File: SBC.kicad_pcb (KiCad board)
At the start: 2 copper layers, 160 x 100.3 mm, 101 parts, among them K1 A17, K10 BNKSEL, K11 16K/32K, K12 INTSEL, K13 RSTSEL, K2 CTS-DSR, K3 RTS-DTR, K4 CTS-DSR, K5 RTS-DTR, K6 A18, K7 128/512, K8 A19, K9 PWR, P1 PARALLEL, P2 POWER, P3 SERIAL, P4 CLK_CPU, P5 CLK_UART, P6 RESET, Q1 2N3906, SW1 RESETSW, U1 16550, U10 74LS243, U11 74LS245, U12 74LS174, U13 74LS174, U14 74LS32, U15 74LS32, U16 74LS32, U17 74LS244, U18 74LS174, U19 8255, U2 27C080, U20 C96ABC, U21 DS1302, U22 MAX232, U23 SRAM_512KO, U24 Z80-CPU, U25 DS1210, U26 74LS06N, U3 74LS08, U4 74LS10, U5 74LS125, U6 74LS139, U7 74LS14, U8 74LS245, U9 74LS245, X1 CRYSTAL

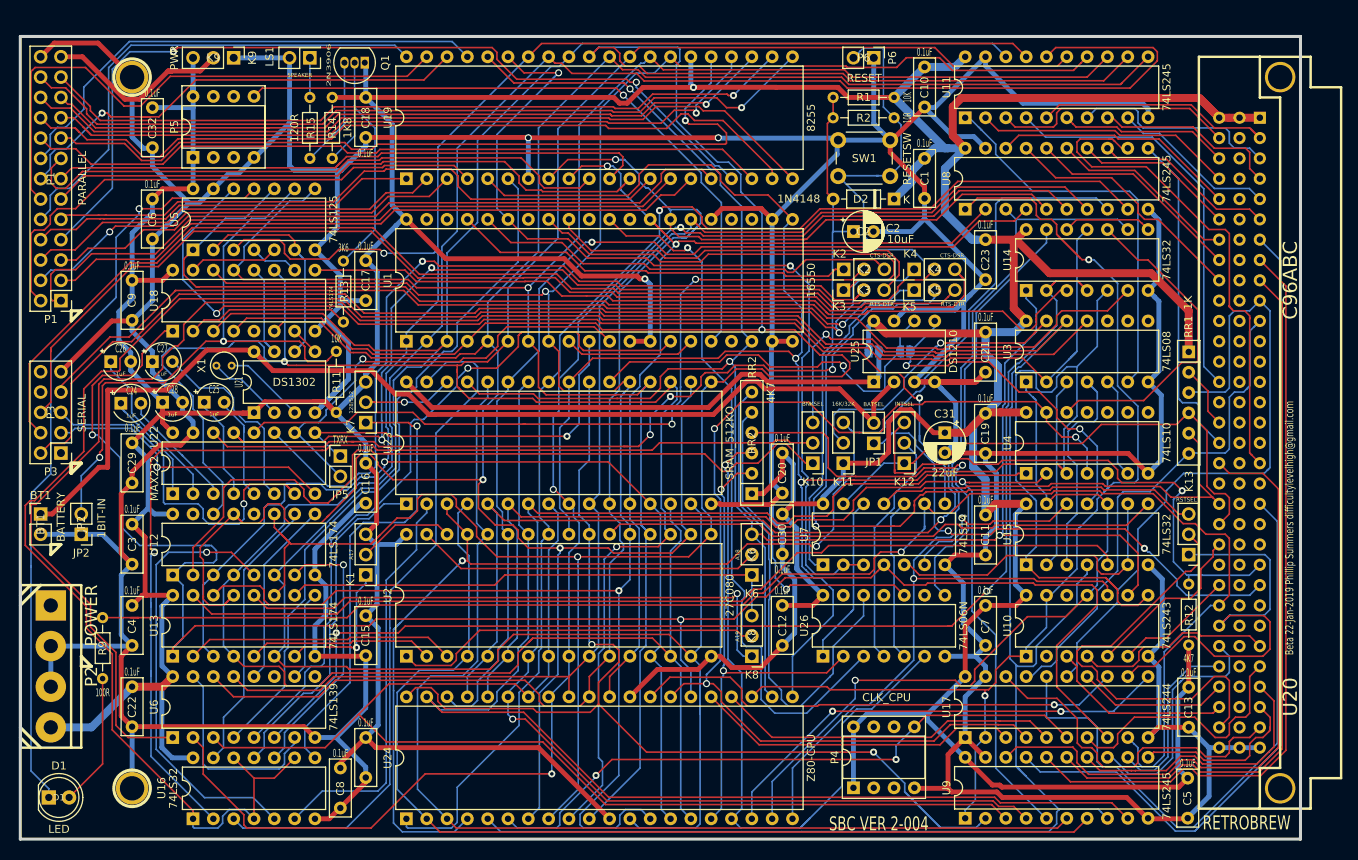
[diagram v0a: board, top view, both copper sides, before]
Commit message: Version G
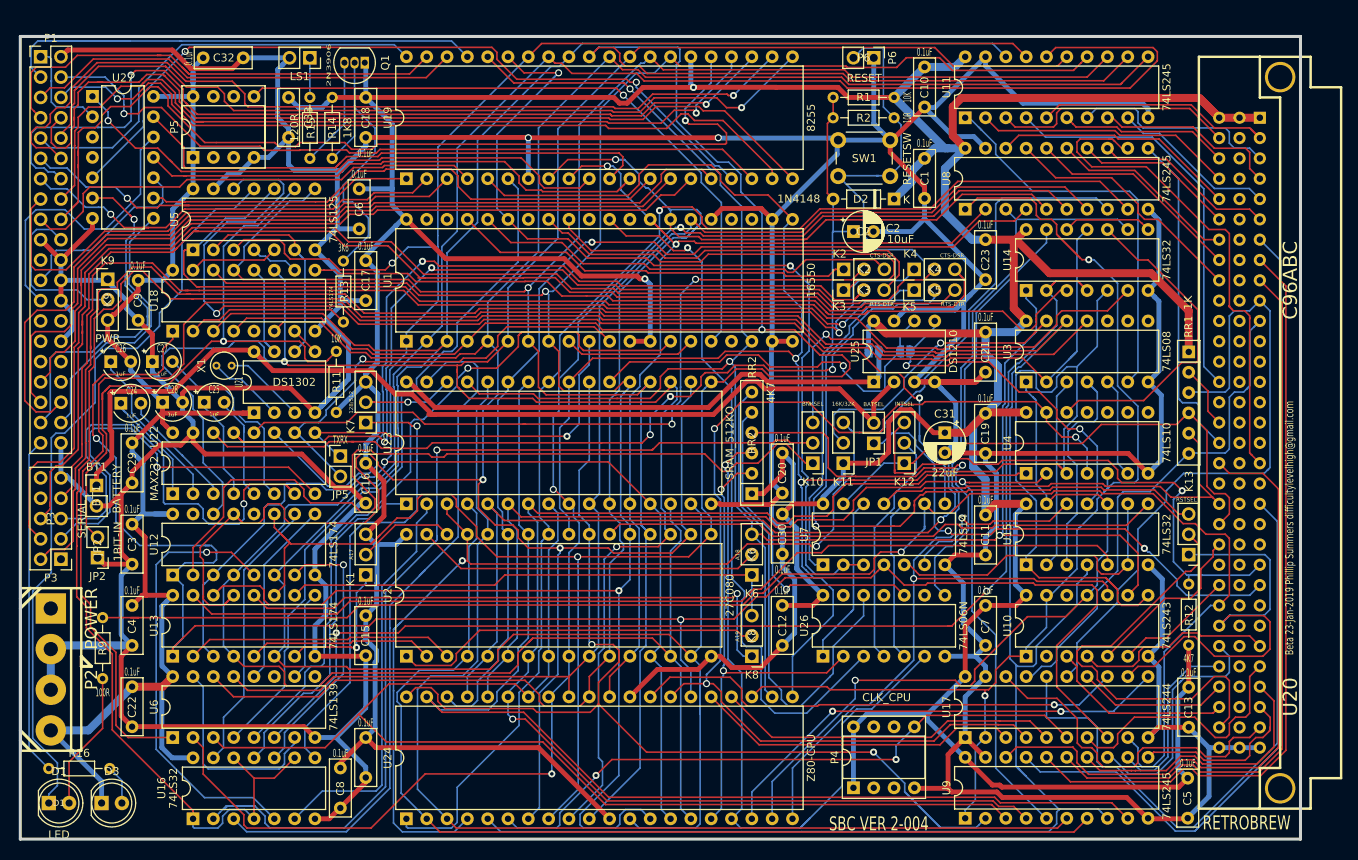
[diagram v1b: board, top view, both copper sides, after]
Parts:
- removed hole1, hole2: CONN_1, 1pin
- added C33: 0.1uF, Capacitor_THT:C_Disc_D7.0mm_W2.5mm_P5.00mm, F.Cu at (111.0, 61.0)
- added D3: LED, LED_THT:LED_D5.0mm, F.Cu at (87.6, 149.2)
- added R16: 470R, Resistor_THT:R_Axial_DIN0204_L3.6mm_D1.6mm_P7.62mm_Horizontal, F.Cu at (81.0, 144.8)
- added U27: 74LS14, Package_DIP:DIP-14_W7.62mm, F.Cu at (86.5, 60.8)
- P1: value PARALLEL -> IDE; footprint Connector_PinHeader_2.54mm:PinHeader_2x13_P2.54mm_Vertical -> Connector_PinHeader_2.54mm:PinHeader_2x20_P2.54mm_Vertical
- moved K9 31.9 mm to (88.4, 83.7), turned to 0 degrees
- moved P1 30.6 mm to (80.0, 55.9), turned to 0 degrees
- moved C6 25.9 mm to (119.8, 72.4)
- moved P3 13.3 mm to (82.5, 118.7)
- moved C32 8.89 mm to (100.3, 56.0), turned to 0 degrees
- moved BT1 7.84 mm to (87.0, 109.5)
- moved JP2 3.56 mm to (87.1, 118.5)
- moved C9 0.76 mm to (92.2, 83.8)
- moved D1 0.70 mm to (81.0, 149.2)
- moved P2 0.38 mm to (81.3, 132.5)
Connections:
- K9 pad 2: /PPWR -> Net-(K9-Pad2)
- P1 pad 1: /PC0 -> /-PC7
- P1 pad 10: /PA4 -> /PB3
- P1 pad 11: /PC5 -> /PA3
- P1 pad 12: /PA5 -> /PB4
- P1 pad 13: /PC6 -> /PA2
- P1 pad 14: /PA6 -> /PB5
- P1 pad 15: /PC7 -> /PA1
- P1 pad 16: /PA7 -> /PB6
- P1 pad 17: /PB7 -> /PA0
- P1 pad 18: /PB0 -> /PB7
- P1 pad 19: /PB6 -> GND
- P1 pad 2: /PA0 -> GND
- P1 pad 20: /PB1 -> Net-(K9-Pad2)
- P1 pad 21: /PB5 -> Net-(P1-Pad21)
- P1 pad 22: /PB2 -> GND
- P1 pad 23: /PB4 -> /-PC5
- P1 pad 24: /PB3 -> GND
- P1 pad 25: /PPWR -> /-PC6
- P1 pad 3: /PC1 -> /PA7
- P1 pad 4: /PA1 -> /PB0
- P1 pad 5: /PC2 -> /PA6
- P1 pad 6: /PA2 -> /PB1
- P1 pad 7: /PC3 -> /PA5
- P1 pad 8: /PA3 -> /PB2
- P1 pad 9: /PC4 -> /PA4
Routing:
- net /-PC3: track 0.00 -> 45.3 mm, vias 0 -> 1
- net Net-(P1-Pad39): track 0.00 -> 42.3 mm
- net GND: track 887.0 -> 926.8 mm
- net /-PC6: track 0.00 -> 36.4 mm
- net /-PC4: track 0.00 -> 34.7 mm
- net /PC2: track 87.0 -> 112.6 mm
- net /-PC5: track 0.00 -> 24.2 mm
- net /PPWR: track 23.9 -> 0.00 mm
- net /DTR: track 116.1 -> 138.1 mm
- net /DSR: track 129.8 -> 151.7 mm
- net Net-(K9-Pad2): track 0.00 -> 21.3 mm
- net /PB5: track 92.8 -> 112.5 mm, vias 1 -> 2
- net /CTS: track 139.6 -> 158.6 mm
- net /RTS: track 137.0 -> 155.5 mm
- net /PB7: track 102.3 -> 119.2 mm
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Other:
- board text added: "Beta 23-Jan-2019 Phillip Summers difficultylevelhigh@gmail.com"
- board text removed: "Beta 22-Jan-2019 Phillip Summers difficultylevelhigh@gmail.com"

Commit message: Version H
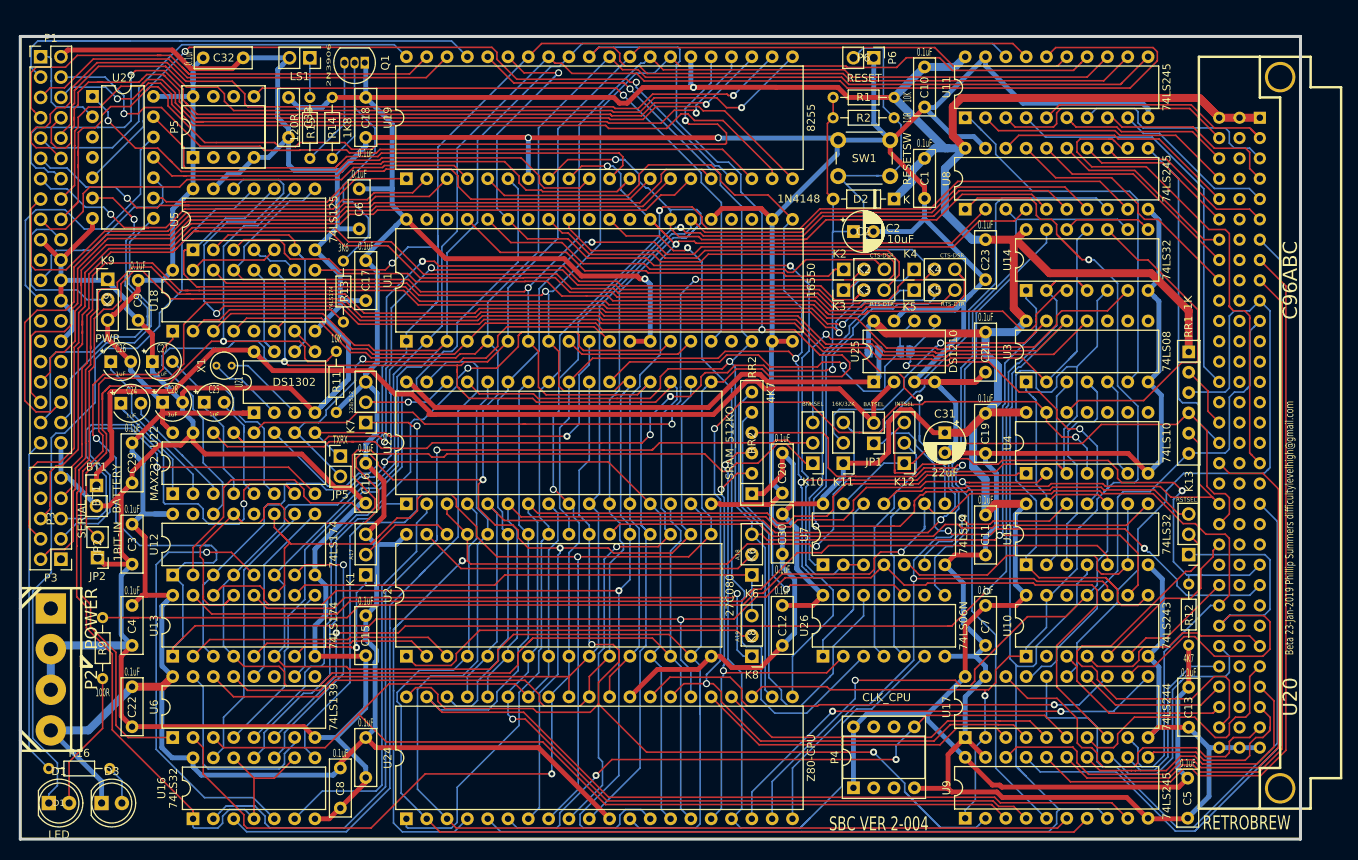
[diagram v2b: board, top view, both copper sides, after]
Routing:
- net VCC: track 852.8 -> 873.0 mm
- net /D0: track 269.8 -> 272.7 mm
- net /CTS: track 158.6 -> 157.8 mm
- net /-PC3: track 45.3 -> 44.5 mm
- net Net-(K10-Pad2): track 122.9 -> 122.3 mm

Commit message: Version I
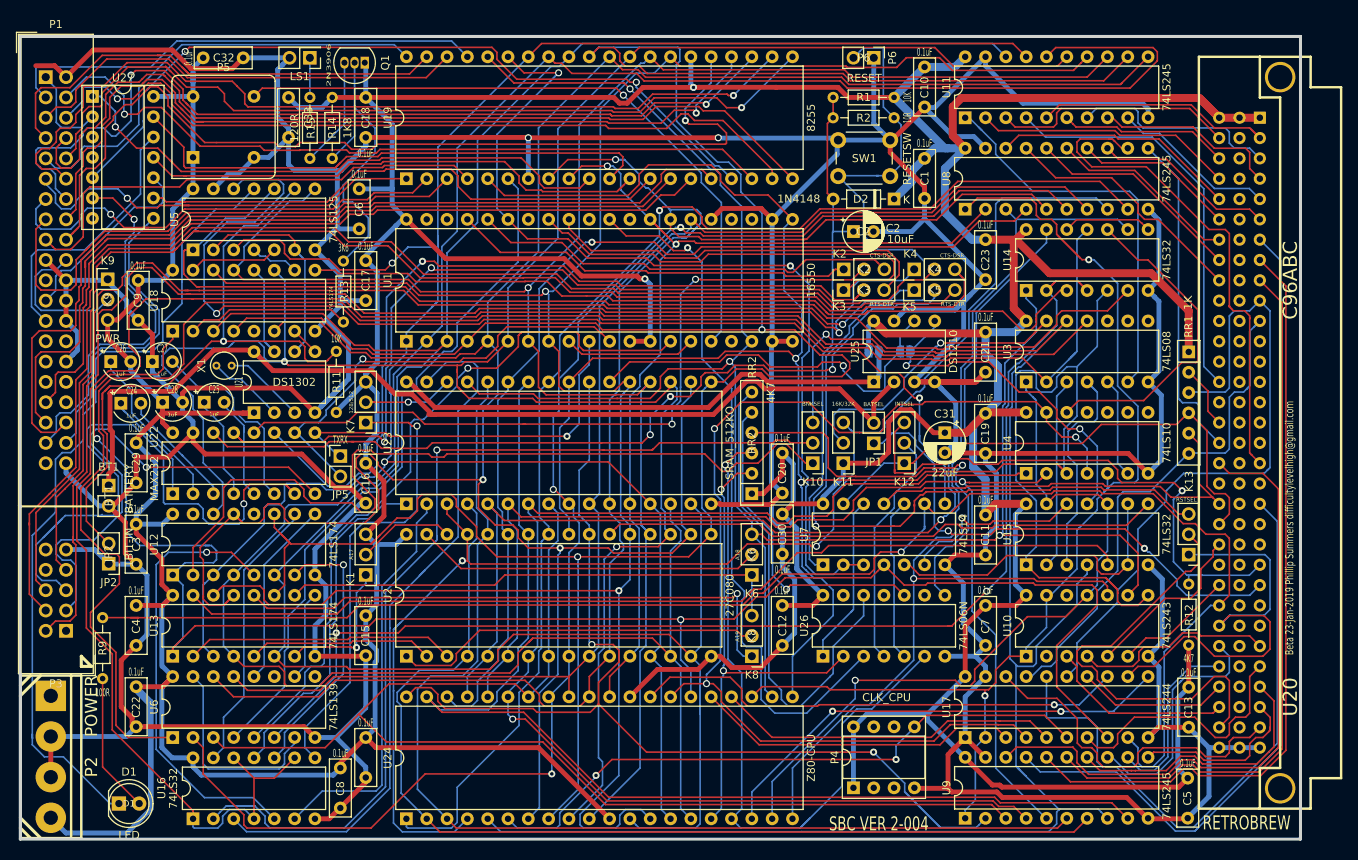
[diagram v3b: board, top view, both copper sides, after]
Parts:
- removed D3: LED, LED_THT:LED_D5.0mm
- removed R16: 470R, Resistor_THT:R_Axial_DIN0204_L3.6mm_D1.6mm_P7.62mm_Horizontal
- P1: footprint Connector_PinHeader_2.54mm:PinHeader_2x20_P2.54mm_Vertical -> Connector_IDC:IDC-Header_2x20_P2.54mm_Vertical
- P3: footprint Connector_PinHeader_2.54mm:PinHeader_2x05_P2.54mm_Vertical -> Connector_IDC:IDC-Header_2x05_P2.54mm_Vertical
- P5: footprint Package_DIP:DIP-8_W7.62mm_Socket -> Oscillator:Oscillator_DIP-8
- U27: footprint Package_DIP:DIP-14_W7.62mm -> Package_DIP:DIP-14_W7.62mm_Socket
- moved P2 10.9 mm to (81.3, 143.4)
- moved P3 8.98 mm to (83.2, 127.6)
- moved D1 8.76 mm to (89.8, 149.2)
- moved P1 2.62 mm to (80.6, 58.4)
- moved JP2 1.59 mm to (88.5, 119.3)
- moved BT1 1.52 mm to (88.5, 109.5)
- moved C22 0.51 mm to (91.9, 134.6)
- moved C29 0.51 mm to (91.9, 104.1)
- moved C3 0.51 mm to (91.9, 114.3)
- moved C4 0.51 mm to (91.9, 124.5)
- turned P5 to 0 degrees
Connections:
- P4 pad 2: Net-(P4-Pad2) -> (no net)
- P4 pad 3: Net-(P4-Pad3) -> (no net)
- P4 pad 6: Net-(P4-Pad6) -> (no net)
- P4 pad 7: Net-(P4-Pad7) -> (no net)
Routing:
- net Net-(P1-Pad39): track 42.3 -> 0.00 mm
- net VCC: track 873.0 -> 894.2 mm
- net /TX: track 59.1 -> 77.3 mm
- net /RX: track 51.1 -> 63.2 mm
- net /PA7: track 71.6 -> 60.6 mm
- net /DSR: track 151.7 -> 160.6 mm
- net /DTR: track 138.1 -> 146.6 mm
- net /CTS: track 157.8 -> 165.8 mm
- net /RTS: track 155.5 -> 162.3 mm
- net Net-(D1-Pad1): track 94.4 -> 101.1 mm
- net Net-(D3-Pad2): track 4.95 -> 0.00 mm
- net /-PC4: track 34.7 -> 39.2 mm
- net /PA2: track 54.1 -> 58.4 mm
- net /PC0: track 100.7 -> 104.2 mm
- net //IOSEL: track 207.2 -> 210.6 mm
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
